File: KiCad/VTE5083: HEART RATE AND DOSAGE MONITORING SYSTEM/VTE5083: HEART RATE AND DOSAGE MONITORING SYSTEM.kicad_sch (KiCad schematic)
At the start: 19 parts, among them J1 Power, J2 Programer, J3 Sensor, SW1 Reset, SW2 Mode, U1 ESP-12E, U2 AMS1117-3.3

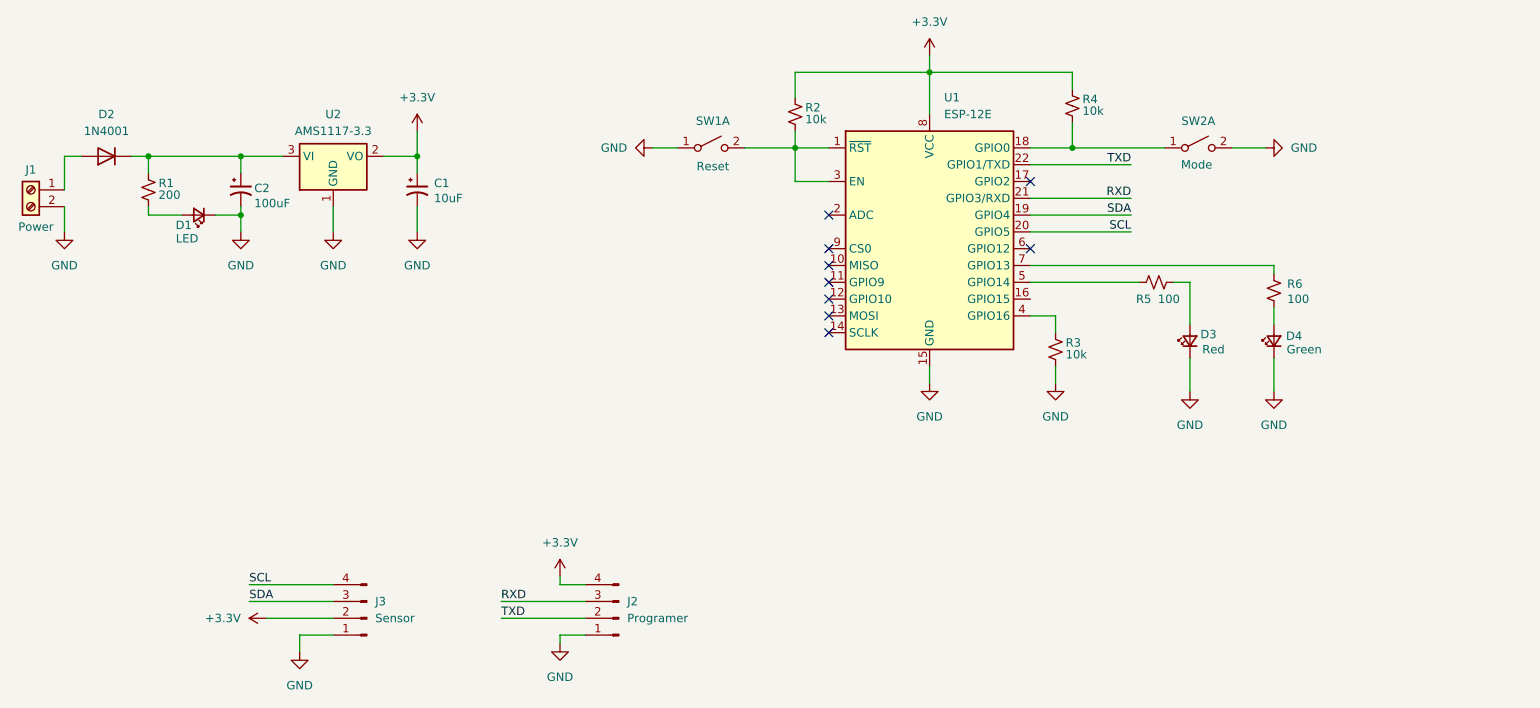
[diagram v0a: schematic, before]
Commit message: Changes
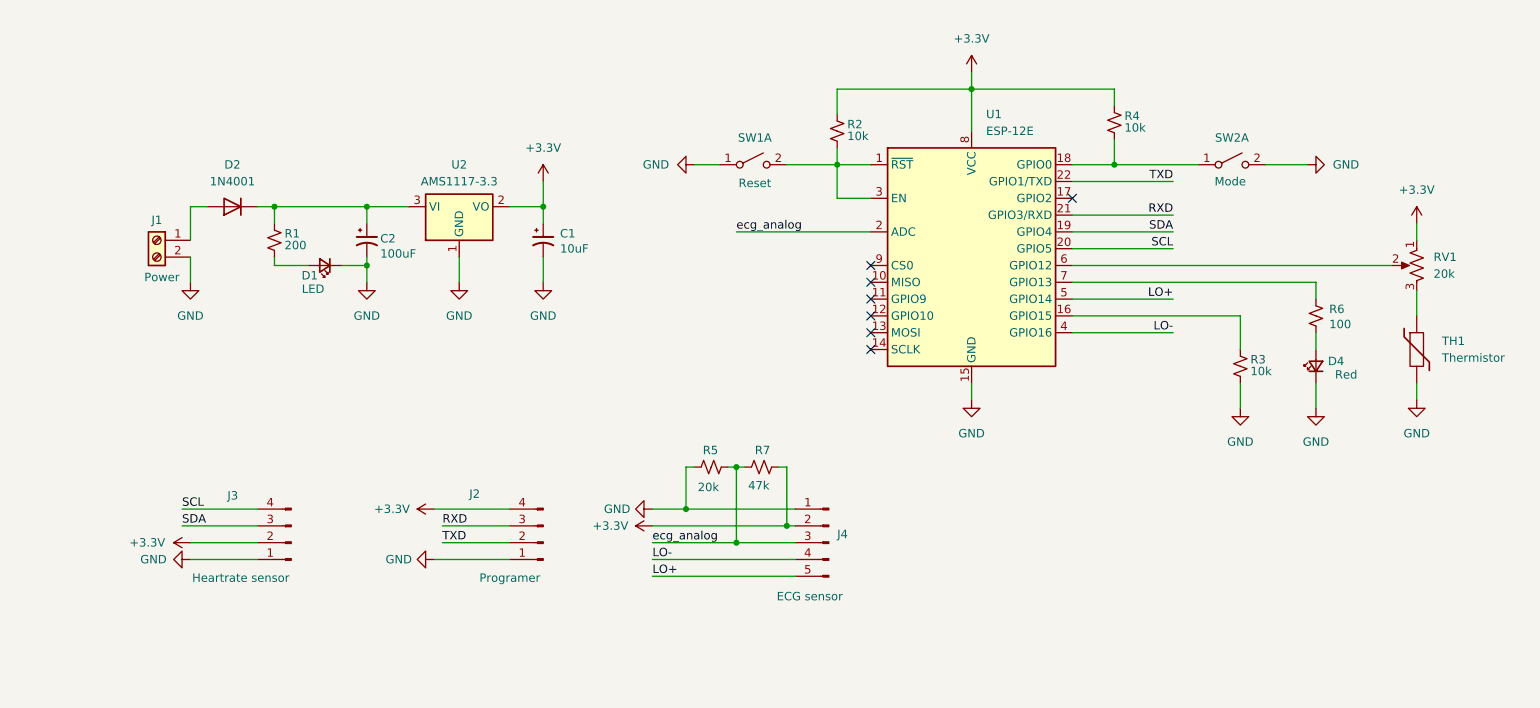
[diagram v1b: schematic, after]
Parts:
- removed D3: Red, LED_THT:LED_D3.0mm_Clear, symbol Device:LED_Small
- added J4: ECG sensor, Connector_PinHeader_2.54mm:PinHeader_1x05_P2.54mm_Vertical, symbol Connector:Conn_01x05_Pin
- added R7: 47k, Resistor_THT:R_Axial_DIN0207_L6.3mm_D2.5mm_P10.16mm_Horizontal, symbol Device:R_Small_US
- added RV1: 20k, Potentiometer_THT:Potentiometer_Runtron_RM-065_Vertical, symbol Device:R_Potentiometer_US
- added TH1: Thermistor, OptoDevice:Osram_SFH225, symbol Device:Thermistor
- D4: value Green -> Red
- J3: value Sensor -> Heartrate sensor
- R5: value 100 -> 20k
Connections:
- net +3.3V: now also J4.2 (Pin_2), R7.1, RV1.1
- net GND: now also R5.2, J4.1 (Pin_1), TH1.2
- net LO+: now reaches U1.5 (GPIO14)
- net LO+: now also J4.5 (Pin_5); no longer R5.1
- net at R3.1: now also U1.16 (GPIO15); no longer U1.4 (GPIO16)
- net ecg_analog: now reaches U1.2 (ADC)
- net ecg_analog: now also R5.1, J4.3 (Pin_3), R7.2
- net at U1.6 (GPIO12): now also RV1.2
- new net: RV1.3, TH1.1
- new net LO-: J4.4 (Pin_4), U1.4 (GPIO16)
- no-connect marks 9 -> 7
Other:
- moved on the sheet: C1, C2, D1, D2, D4, J1, J2, J3, R1, R2, R3, R4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
